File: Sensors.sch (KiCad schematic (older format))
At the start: 4 parts, among them U701 BNO055, U702 DPS422XTSA1, U703 MCP3208, U704 TXB0108PWR

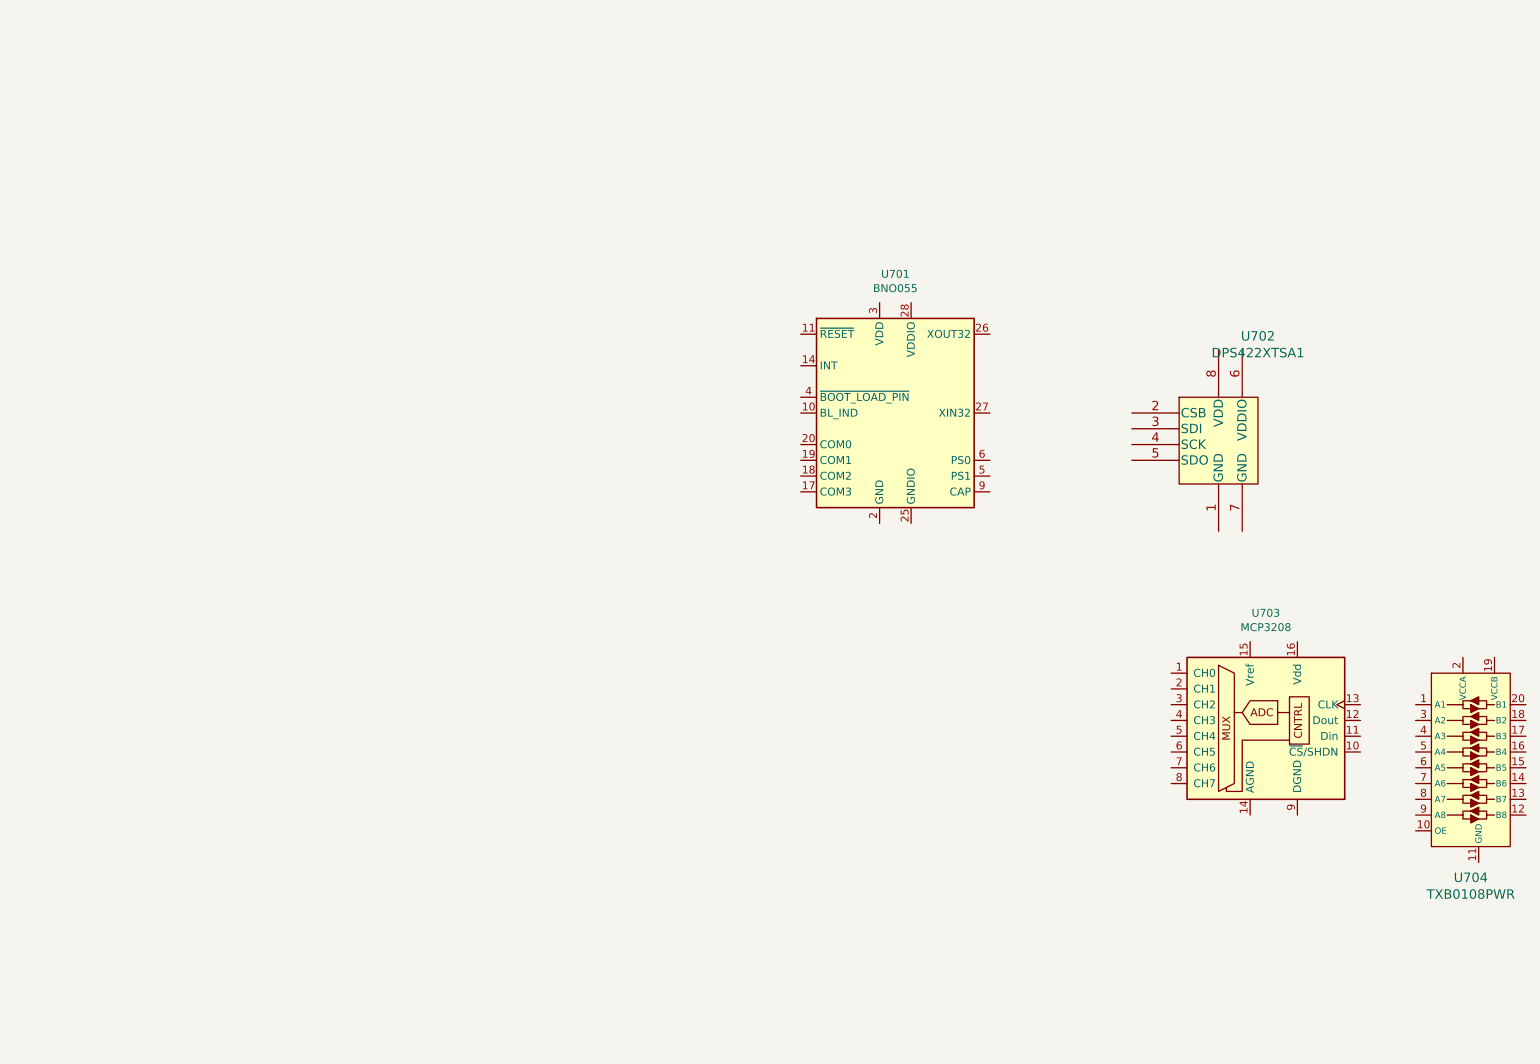
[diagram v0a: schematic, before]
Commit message: Finished v0.1 of power, and v0.1 of sensors.
Signed-off-by: Jan Mart Liewes <Eldalote.Electronics@gmail.com>
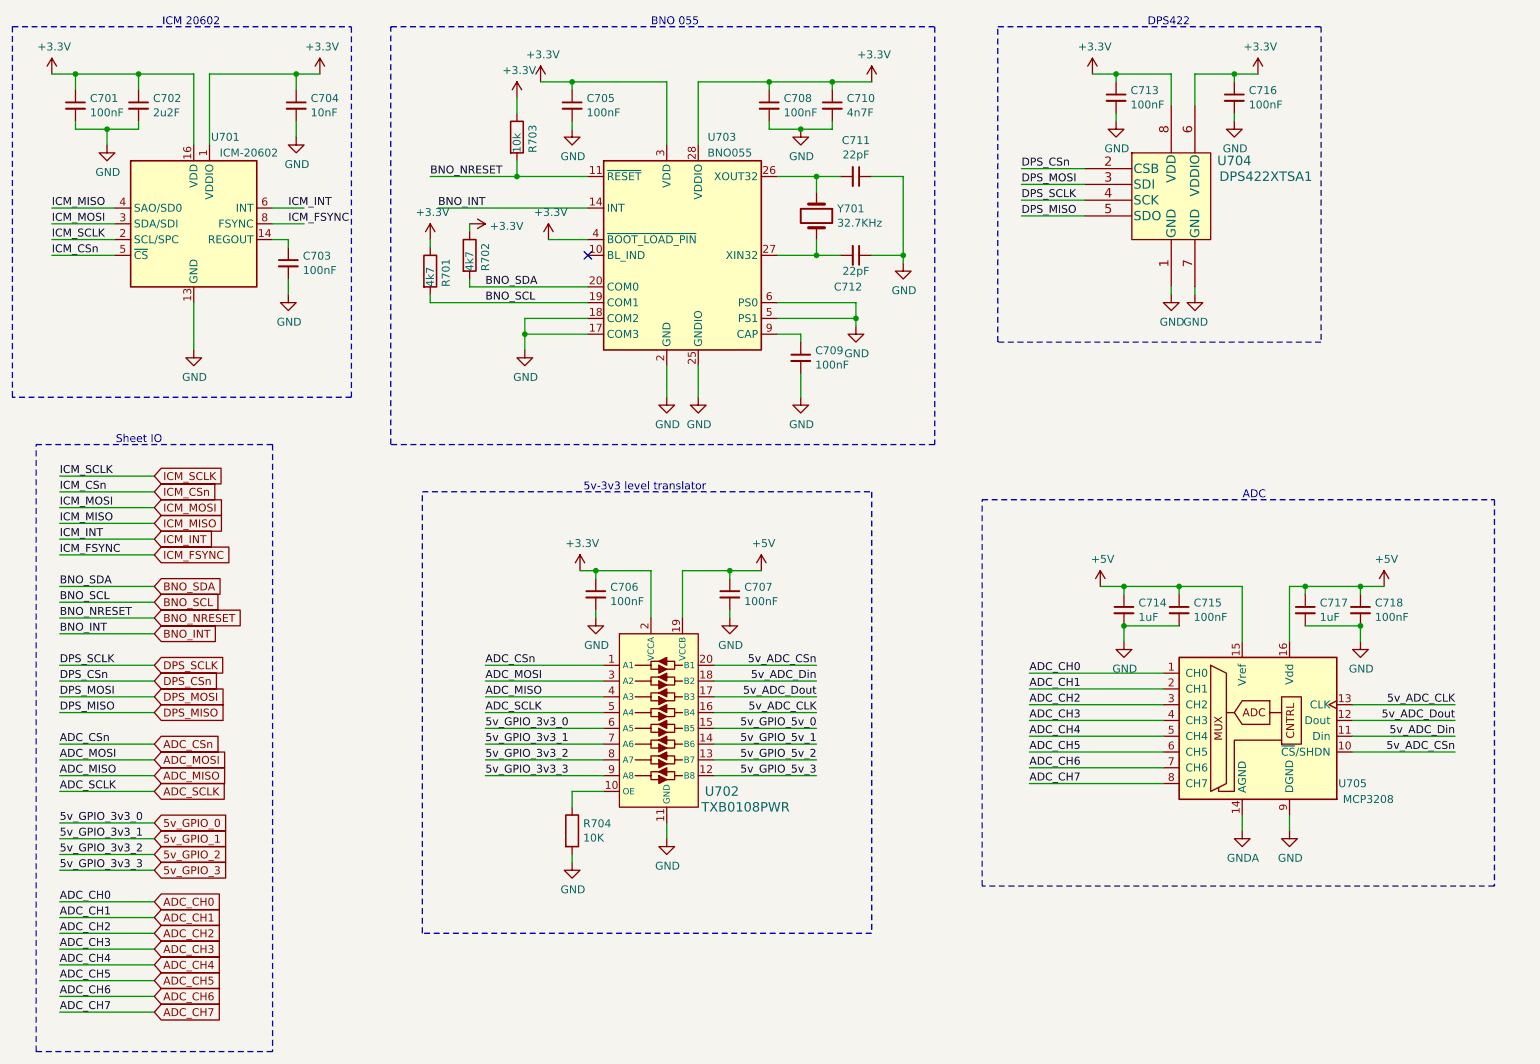
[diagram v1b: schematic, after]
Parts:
- added C701, C703, C705, C708, C709, C713, C716: 100nF, Capacitor_SMD:C_0402_1005Metric, symbol Device:C_Small
- added C702: 2u2F, Capacitor_SMD:C_0603_1608Metric, symbol Device:C_Small
- added C704: 10nF, Capacitor_SMD:C_0402_1005Metric, symbol Device:C_Small
- added C706, C707, C715, C718: 100nF, Capacitor_SMD:C_0805_2012Metric_Pad1.15x1.40mm_HandSolder, symbol Device:C_Small
- added C710: 4n7F, Capacitor_SMD:C_0603_1608Metric, symbol Device:C_Small
- added C711, C712: 22pF, Capacitor_SMD:C_0603_1608Metric, symbol Device:C_Small
- added C714, C717: 1uF, Capacitor_SMD:C_0805_2012Metric_Pad1.15x1.40mm_HandSolder, symbol Device:C_Small
- added R701, R702: 4k7, Resistor_SMD:R_0402_1005Metric, symbol Device:R
- added R703: 10k, Resistor_SMD:R_0402_1005Metric, symbol Device:R
- added R704: 10K, Resistor_SMD:R_0805_2012Metric_Pad1.15x1.40mm_HandSolder, symbol Device:R
- added U701: ICM-20602, Package_LGA:LGA-16_3x3mm_P0.5mm_LayoutBorder3x5y, symbol Sensor_Motion:ICM-20602
- added Y701: 32.7KHz, Crystal:Crystal_SMD_3215-2Pin_3.2x1.5mm, symbol Device:Crystal
- renumbered U704 to U702, U701 to U703, U702 to U704, U703 to U705
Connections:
- net BNO_NRESET: now reaches U703.11 (~RESET)
- net BNO_NRESET: now also R703.2
- net BNO_INT: now reaches U703.14 (INT)
- net GND: now reaches U703.15 (GNDIO), U703.16 (GNDIO), U703.25 (GNDIO)
- net GND: now also U702.11 (GND), U703.17 (COM3), U703.18 (COM2), U703.2 (GND), U703.5 (PS1), U703.6 (PS0), U704.1 (GND), U704.7 (GND), U705.9 (DGND), C701.2, C702.2, C703.2, C704.2, C705.2, C706.2, C707.2, C708.2, C709.2, C710.2, C711.1, C712.1, C713.2, C714.2, C715.2, C716.2, C717.2, C718.2, R704.2, U701.10 (GND), U701.11 (GND), U701.12 (GND), U701.13 (GND), U701.15 (GND), U701.9 (GND)
- net BNO_SCL: now reaches U703.19 (COM1)
- net BNO_SCL: now also R701.2
- net BNO_SDA: now reaches U703.20 (COM0)
- net BNO_SDA: now also R702.2
- net at U703.26 (XOUT32): now also C711.2, Y701.1
- net at U703.27 (XIN32): now also C712.2, Y701.2
- net +3V3: now reaches U703.28 (VDDIO)
- net +3V3: now also U702.2 (VCCA), U703.3 (VDD), U703.4 (~BOOT_LOAD_PIN), U704.6 (VDDIO), U704.8 (VDD), C701.1, C702.1, C704.1, C705.1, C706.1, C708.1, C710.1, C713.1, C716.1, R701.1, R702.1, R703.1, U701.1 (VDDIO), U701.16 (VDD)
- net at U703.9 (CAP): now also C709.1
- net DPS_CSn: now reaches U704.2 (CSB)
- net DPS_MOSI: now reaches U704.3 (SDI)
- net DPS_SCLK: now reaches U704.4 (SCK)
- net DPS_MISO: now reaches U704.5 (SDO)
- net ADC_CH0: now reaches U705.1 (CH0)
- net 5v_ADC_CSn: now reaches U705.10 (~CS~/SHDN)
- net 5v_ADC_CSn: now also U702.20 (B1)
- net 5v_ADC_Din: now reaches U705.11 (Din)
- net 5v_ADC_Din: now also U702.18 (B2)
- net 5v_ADC_Dout: now reaches U705.12 (Dout)
- net 5v_ADC_Dout: now also U702.17 (B3)
- net 5v_ADC_CLK: now reaches U705.13 (CLK)
- net 5v_ADC_CLK: now also U702.16 (B4)
- net GNDA: now reaches U705.14 (AGND)
- net +5V: now reaches U705.15 (Vref)
- net +5V: now also U702.19 (VCCB), U705.16 (Vdd), C707.1, C714.1, C715.1, C717.1, C718.1
- net ADC_CH1: now reaches U705.2 (CH1)
- net ADC_CH2: now reaches U705.3 (CH2)
- net ADC_CH3: now reaches U705.4 (CH3)
- net ADC_CH4: now reaches U705.5 (CH4)
- net ADC_CH5: now reaches U705.6 (CH5)
- net ADC_CH6: now reaches U705.7 (CH6)
- net ADC_CH7: now reaches U705.8 (CH7)
- net ADC_CSn: now reaches U702.1 (A1)
- net at U702.10 (OE): now also R704.1
- net 5v_GPIO_5v_3: now reaches U702.12 (B8)
- net 5v_GPIO_5v_2: now reaches U702.13 (B7)
- net 5v_GPIO_5v_1: now reaches U702.14 (B6)
- net 5v_GPIO_5v_0: now reaches U702.15 (B5)
- net ADC_MOSI: now reaches U702.3 (A2)
- net ADC_MISO: now reaches U702.4 (A3)
- net ADC_SCLK: now reaches U702.5 (A4)
- net 5v_GPIO_0: now reaches U702.6 (A5)
- net 5v_GPIO_1: now reaches U702.7 (A6)
- net 5v_GPIO_2: now reaches U702.8 (A7)
- net 5v_GPIO_3: now reaches U702.9 (A8)
- new net: C703.1, U701.14 (REGOUT)
- new net ICM_CSn: U701.5 (~CS)
- new net ICM_FSYNC: U701.8 (FSYNC)
- new net ICM_INT: U701.6 (INT)
- new net ICM_MISO: U701.4 (SAO/SD0)
- new net ICM_MOSI: U701.3 (SDA/SDI)
- new net ICM_SCLK: U701.2 (SCL/SPC)
- no-connect marks 0 -> 1
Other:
- note added: "5v-3v3 level translator"
- note added: "ADC"
- note added: "BNO 055"
- note added: "DPS422"
- note added: "ICM 20602"
- note added: "Sheet IO"
- moved on the sheet: U702, U703, U704, U705
